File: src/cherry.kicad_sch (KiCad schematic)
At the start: 9 parts, among them J1 USB_C, J2 GPIO_Header, U1 FT2232HL, U2 ICE40LP8K-CM81, U3 W25Q32JVSSIQ, U4 AMS1117-3.3, U5 AP2112K-1.2, Y1 12MHz

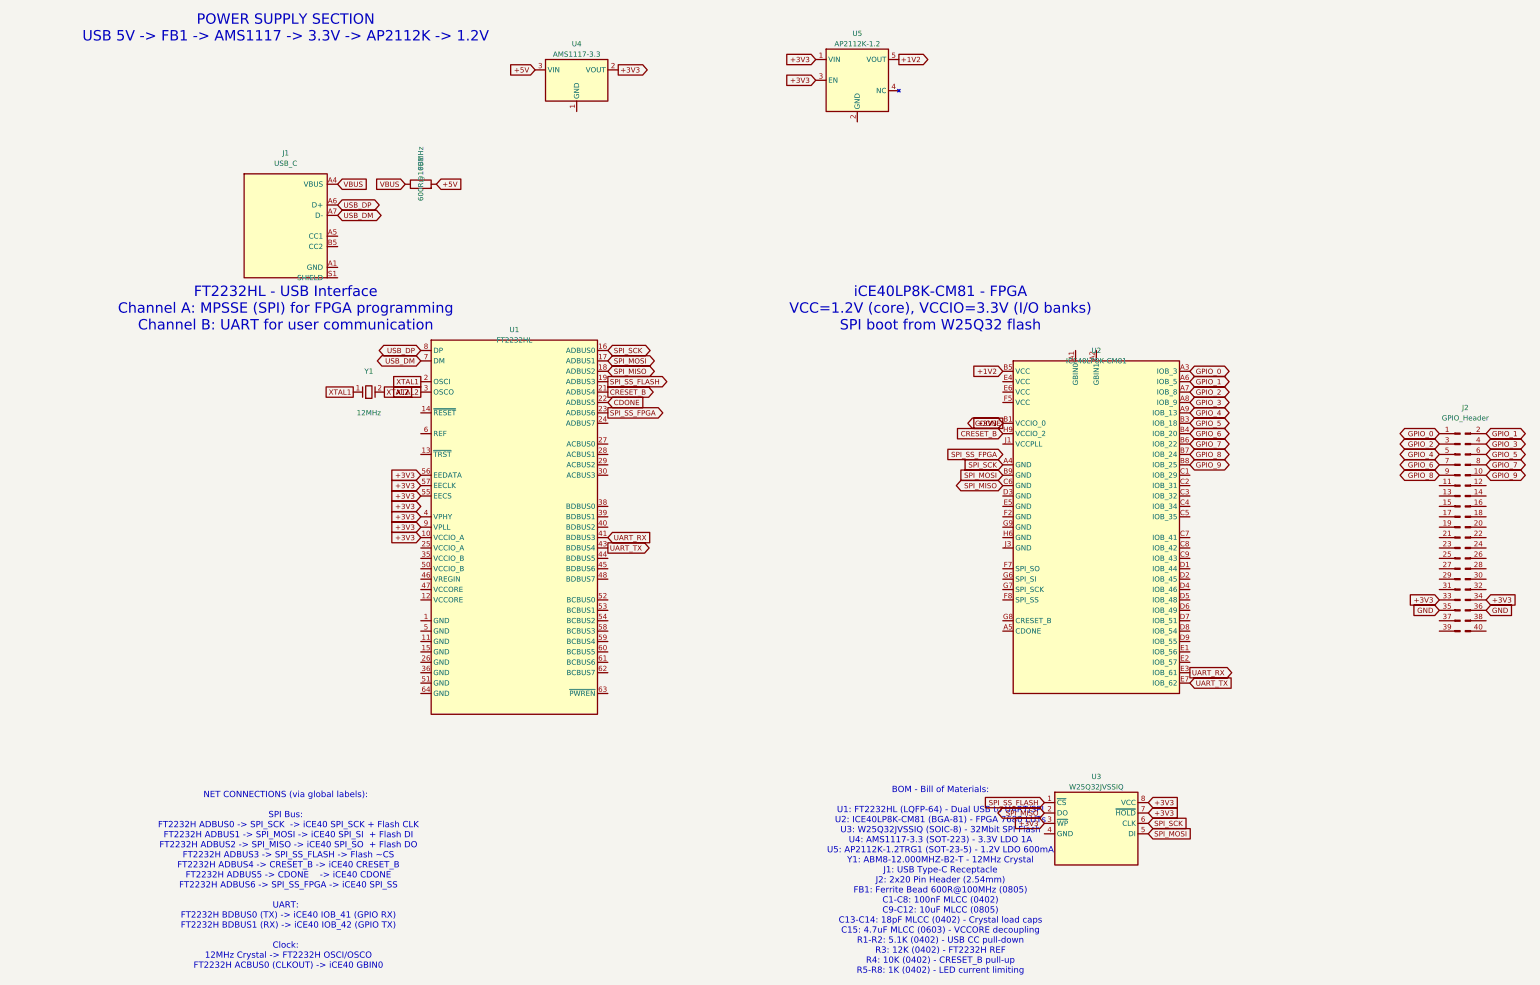
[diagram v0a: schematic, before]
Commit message: chore
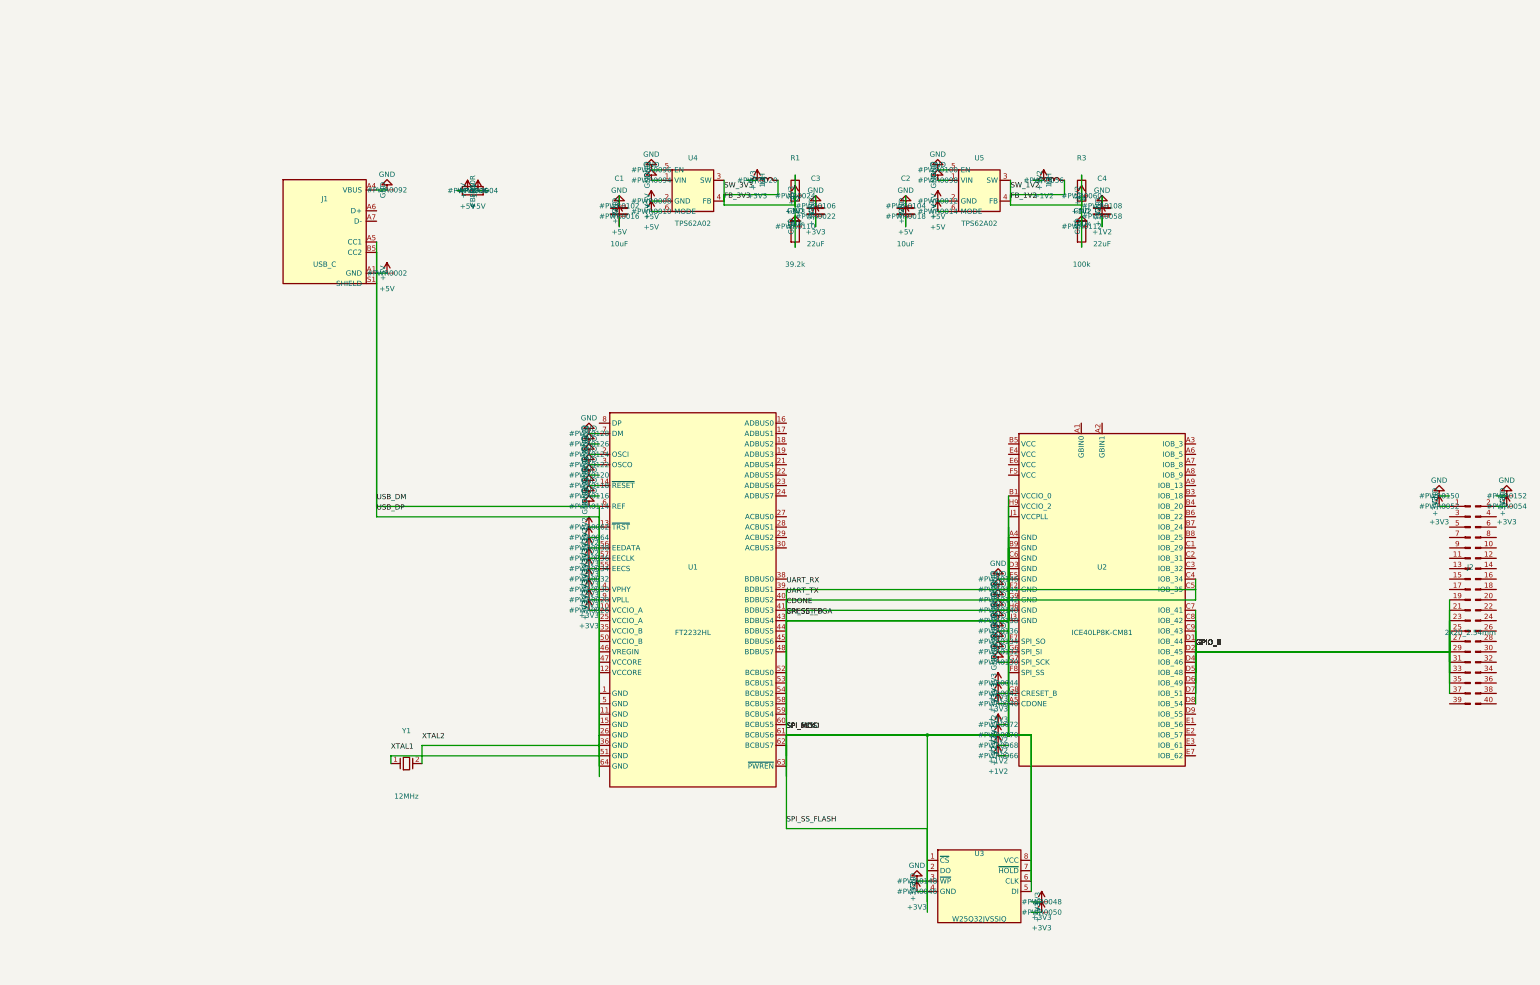
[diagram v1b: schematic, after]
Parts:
- added C1, C2: 10uF, symbol Cherry:C
- added C3, C4: 22uF, symbol Cherry:C
- added L1, L2: 1uH, symbol Cherry:L
- added R1: 180k, symbol Cherry:R
- added R2: 39.2k, symbol Cherry:R
- added R3, R4: 100k, symbol Cherry:R
- FB1: value 600R@100MHz -> FB_600R; footprint Inductor_SMD:L_0805_2012Metric -> (none); symbol Device:Ferrite_Bead -> Cherry:Ferrite_Bead
- J1: footprint Connector_USB:USB_C_Receptacle_GCT_USB4125 -> (none); symbol Connector:USB_C_Receptacle_USB2.0 -> Cherry:USB_C_Receptacle_USB2.0
- J2: value GPIO_Header -> 2x20_2.54mm; footprint Connector_PinHeader_2.54mm:PinHeader_2x20_P2.54mm_Vertical -> (none); symbol Connector_Generic:Conn_02x20_Odd_Even -> Cherry:Conn_02x20_Odd_Even
- U1: footprint Package_QFP:LQFP-64_10x10mm_P0.5mm -> (none)
- U2: footprint Package_BGA:BGA-81_9x9_8.0x8.0mm_P0.8mm -> (none)
- U3: footprint Package_SO:SOIC-8_3.9x4.9mm_P1.27mm -> (none)
- U4: value AMS1117-3.3 -> TPS62A02; footprint Package_TO_SOT_SMD:SOT-223-3_TabPin2 -> (none); symbol Cherry:AMS1117-3.3 -> Cherry:TPS62A02
- U5: value AP2112K-1.2 -> TPS62A02; footprint Package_TO_SOT_SMD:SOT-23-5 -> (none); symbol Cherry:AP2112K-1.2 -> Cherry:TPS62A02
- Y1: footprint Crystal:Crystal_SMD_3215-2Pin_3.2x1.5mm -> (none); symbol Device:Crystal -> Cherry:Crystal
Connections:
- net +1V2: now also J1.A4 (VBUS), J2.1 (Pin_1), J2.2 (Pin_2), U1.10 (VCCIO_A), U1.13 (~{TRST}), U1.14 (~{RESET}), U1.2 (OSCI), U1.3 (OSCO), U1.4 (VPHY), U1.55 (EECS), U1.56 (EEDATA), U1.57 (EECLK), U1.6 (REF), U1.7 (DM), U1.9 (VPLL), U2.A5 (CDONE), U2.E5 (GND), U2.F2 (GND), U2.F7 (SPI_SO), U2.G6 (SPI_SI), U2.G7 (SPI_SCK), U2.G8 (CRESET_B), U2.G9 (GND), U2.H6 (GND), U2.J3 (GND), U3.3 (~{WP}), U3.4 (GND), U4.1 (VIN), U4.3 (SW), U4.4 (FB), U4.5 (EN), U5.1 (VIN), U5.3 (SW), U5.4 (FB), C1.1, C2.1, C3.1, C3.2, C4.1, C4.2, L1.1, L1.2, L2.1, L2.2, R1.1, R1.2, R2.1, R2.2, R3.1, R3.2, R4.1, R4.2; no longer U2.B5 (VCC)
- net +5V: now also FB1.1, J1.A1 (GND), U4.2 (GND), U4.6 (MODE), U5.2 (GND), U5.6 (MODE), C1.2, C2.2; no longer U4.3 (VIN)
- net GPIO_0: now also J2.19 (Pin_19), J2.21 (Pin_21), J2.23 (Pin_23), J2.25 (Pin_25), J2.27 (Pin_27), J2.29 (Pin_29), J2.31 (Pin_31), J2.33 (Pin_33), J2.35 (Pin_35), J2.37 (Pin_37), U2.C7 (IOB_41), U2.C8 (IOB_42), U2.C9 (IOB_43), U2.D1 (IOB_44), U2.D2 (IOB_45), U2.D4 (IOB_46), U2.D5 (IOB_48), U2.D6 (IOB_49), U2.D7 (IOB_51), U2.D8 (IOB_54); no longer J2.1 (Pin_1), U2.A3 (IOB_3)
- net UART_RX: no longer U1.41 (BDBUS3), U2.E3 (IOB_61)
- net USB_DM: now also J1.A5 (CC1), J1.B5 (CC2), U1.26 (GND), U1.36 (GND), U1.64 (GND), Y1.1, Y1.2; no longer J1.A7 (D-), U1.7 (DM)
- net XTAL1: no longer U1.2 (OSCI), Y1.1
- net XTAL2: no longer U1.3 (OSCO), Y1.2
- net CDONE: now reaches U1.59 (BCBUS4)
- net CDONE: now also U1.41 (BDBUS3), U1.43 (BDBUS4), U1.60 (BCBUS5), U1.61 (BCBUS6), U1.62 (BCBUS7), U1.63 (~{PWREN}), U2.A4 (GND), U2.B1 (VCCIO_0), U2.B9 (GND), U2.C4 (IOB_34), U2.C5 (IOB_35), U2.C6 (GND), U2.H9 (VCCIO_2), U3.5 (DI), U3.6 (CLK)
- removed net +3V3: J2.33 (Pin_33), J2.34 (Pin_34), U1.10 (VCCIO_A), U1.22 (ADBUS5), U1.4 (VPHY), U1.55 (EECS), U1.56 (EEDATA), U1.57 (EECLK), U1.9 (VPLL), U2.B1 (VCCIO_0), U3.3 (~{WP}), U3.7 (~{HOLD}), U3.8 (VCC), U4.2 (VOUT), U5.1 (VIN), U5.3 (EN)
- net CRESET_B: no longer names the net of U1.21 (ADBUS4)
- net CRESET_B: no longer U2.H9 (VCCIO_2)
- net GND: no longer names the net of J2.36 (Pin_36)
- net GND: no longer J2.35 (Pin_35)
- net GPIO_1: no longer names the net of U2.A6 (IOB_5)
- net GPIO_1: no longer J2.2 (Pin_2)
- net GPIO_2: no longer names the net of U2.A7 (IOB_8)
- net GPIO_2: no longer J2.3 (Pin_3)
- net GPIO_3: no longer names the net of U2.A8 (IOB_9)
- net GPIO_3: no longer J2.4 (Pin_4)
- net GPIO_4: no longer names the net of U2.A9 (IOB_13)
- net GPIO_4: no longer J2.5 (Pin_5)
- net GPIO_5: no longer names the net of U2.B3 (IOB_18)
- net GPIO_5: no longer J2.6 (Pin_6)
- net GPIO_6: no longer names the net of U2.B4 (IOB_20)
- net GPIO_6: no longer J2.7 (Pin_7)
- net GPIO_7: no longer names the net of U2.B6 (IOB_22)
- net GPIO_7: no longer J2.8 (Pin_8)
- net GPIO_8: no longer names the net of U2.B7 (IOB_24)
- net GPIO_8: no longer J2.9 (Pin_9)
- net GPIO_9: no longer names the net of U2.B8 (IOB_25)
- net GPIO_9: no longer J2.10 (Pin_10)
- removed net SPI_MISO: U1.18 (ADBUS2), U2.C6 (GND), U3.2 (DO)
- removed net SPI_MOSI: U1.17 (ADBUS1), U2.B9 (GND), U3.5 (DI)
- removed net SPI_SCK: U1.16 (ADBUS0), U2.A4 (GND), U3.6 (CLK)
- net SPI_SS_FLASH: no longer names the net of U1.19 (ADBUS3)
- net SPI_SS_FLASH: no longer U3.1 (~{CS})
- net SPI_SS_FPGA: no longer names the net of U1.23 (ADBUS6)
- net UART_TX: no longer names the net of U2.E7 (IOB_62)
- net UART_TX: no longer U1.43 (BDBUS4)
- net USB_DP: no longer names the net of J1.A6 (D+)
- net USB_DP: no longer U1.8 (DP)
- removed net VBUS: FB1.1, J1.A4 (VBUS)
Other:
- note removed: "BOM - Bill of Materials: U1: FT2232HL (LQFP-64) - Dual USB to UART/SPI U2: ICE40LP8K-CM81 (BGA-81) - FPGA 7680 LUTs U3: W25Q32JVSSIQ (SOIC-8) - 32Mbit SPI Flash U4: AMS1117-3.3 (SOT-223) - 3.3V LDO 1A U5: AP2112K-1.2TRG1 (SOT-23-5) - 1.2V LDO 600mA Y1: ABM8-12.000MHZ-B2-T - 12MHz Crystal J1: USB Type-C Receptacle J2: 2x20 Pin Header (2.54mm) FB1: Ferrite Bead 600R@100MHz (0805) C1-C8: 100nF MLCC 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"
- note removed: "FT2232HL - USB Interface Channel A: MPSSE (SPI) for FPGA programming Channel B: UART for user communication"
- note removed: "NET CONNECTIONS (via global labels): SPI Bus: FT2232H ADBUS0 -> SPI_SCK -> iCE40 SPI_SCK + Flash CLK FT2232H ADBUS1 -> SPI_MOSI -> iCE40 SPI_SI + Flash DI FT2232H ADBUS2 -> SPI_MISO -> iCE40 SPI_SO + Flash DO FT2232H ADBUS3 -> SPI_SS_FLASH -> Flash ~CS FT2232H ADBUS4 -> CRESET_B -> iCE40 CRESET_B FT2232H ADBUS5 -> CDONE -> iCE40 CDONE FT2232H ADBUS6 -> SPI_SS_FPGA -> iCE40 SPI_SS UART: FT2232H BD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"
- note removed: "POWER SUPPLY SECTION USB 5V -> FB1 -> AMS1117 -> 3.3V -> AP2112K -> 1.2V"
- note removed: "iCE40LP8K-CM81 - FPGA VCC=1.2V (core), VCCIO=3.3V (I/O banks) SPI boot from W25Q32 flash"
- moved on the sheet: FB1, J1, J2, U1, U2, U3, Y1
